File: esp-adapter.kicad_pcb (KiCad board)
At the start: 2 copper layers, 16 x 19.6 mm, 4 parts, among them J1 Conn_01x11_Male, J2 Conn_01x11_Male, J3 Conn_01x02_Male, U1 ESP-07

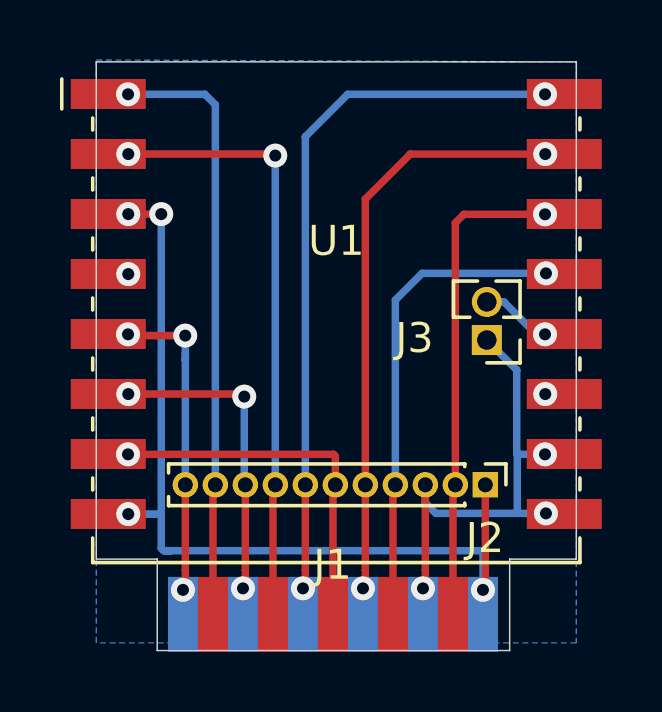
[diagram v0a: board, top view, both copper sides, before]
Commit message: fix TX RX swap
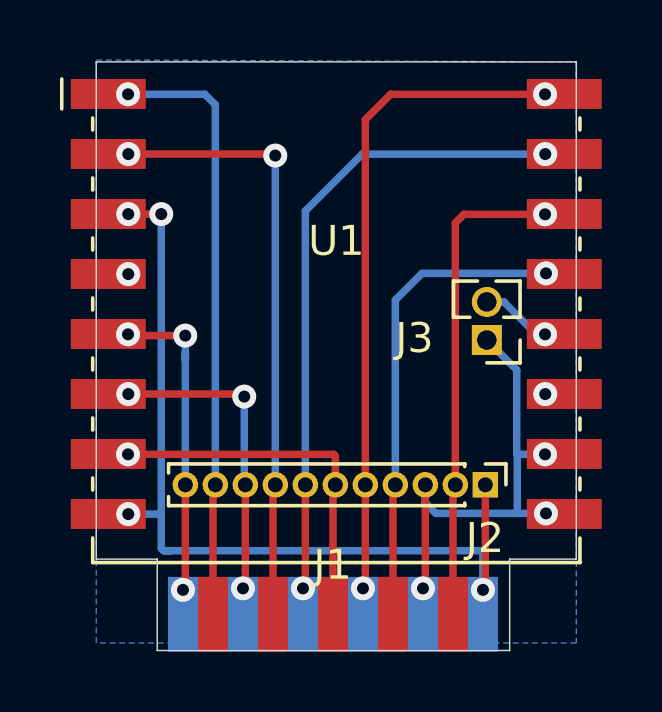
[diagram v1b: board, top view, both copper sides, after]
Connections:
- U1 pad 15: RXD0 -> TXD0
- U1 pad 16: TXD0 -> RXD0
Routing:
- net RXD0: track 21.6 -> 24.0 mm
- net TXD0: track 25.7 -> 23.4 mm

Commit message: Revert "fix TX RX swap"
This reverts commit 031c61bf6d1d21104408cedd763a9be0f04462ce.
For explanation see issue #2 .
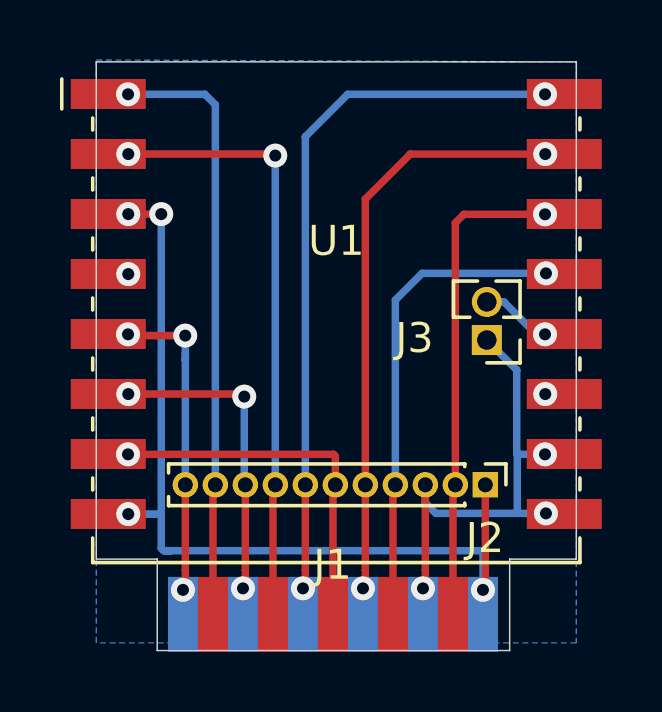
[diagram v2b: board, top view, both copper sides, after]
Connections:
- U1 pad 15: TXD0 -> RXD0
- U1 pad 16: RXD0 -> TXD0
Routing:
- net RXD0: track 24.0 -> 21.6 mm
- net TXD0: track 23.4 -> 25.7 mm
